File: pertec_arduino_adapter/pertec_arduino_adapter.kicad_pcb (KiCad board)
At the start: 2 copper layers, 88.9 x 78.7 mm, 19 parts, among them J1 Conn_02x25_Odd_Even, J2 Conn_02x25_Odd_Even, J3 POWER, J4 ANALOGL, J5 ANALOGH, J6 Conn_02x18_Odd_Even, J7 IOH, J8 IOL, J9 UART, U1 SN74AVC8T245PW, U2 SN74AVC8T245PW, U3 SN74AVC8T245PW, U4 SN74AVC8T245PW, U5 SN74AVC8T245PW, U6 SN74AVC8T245PW

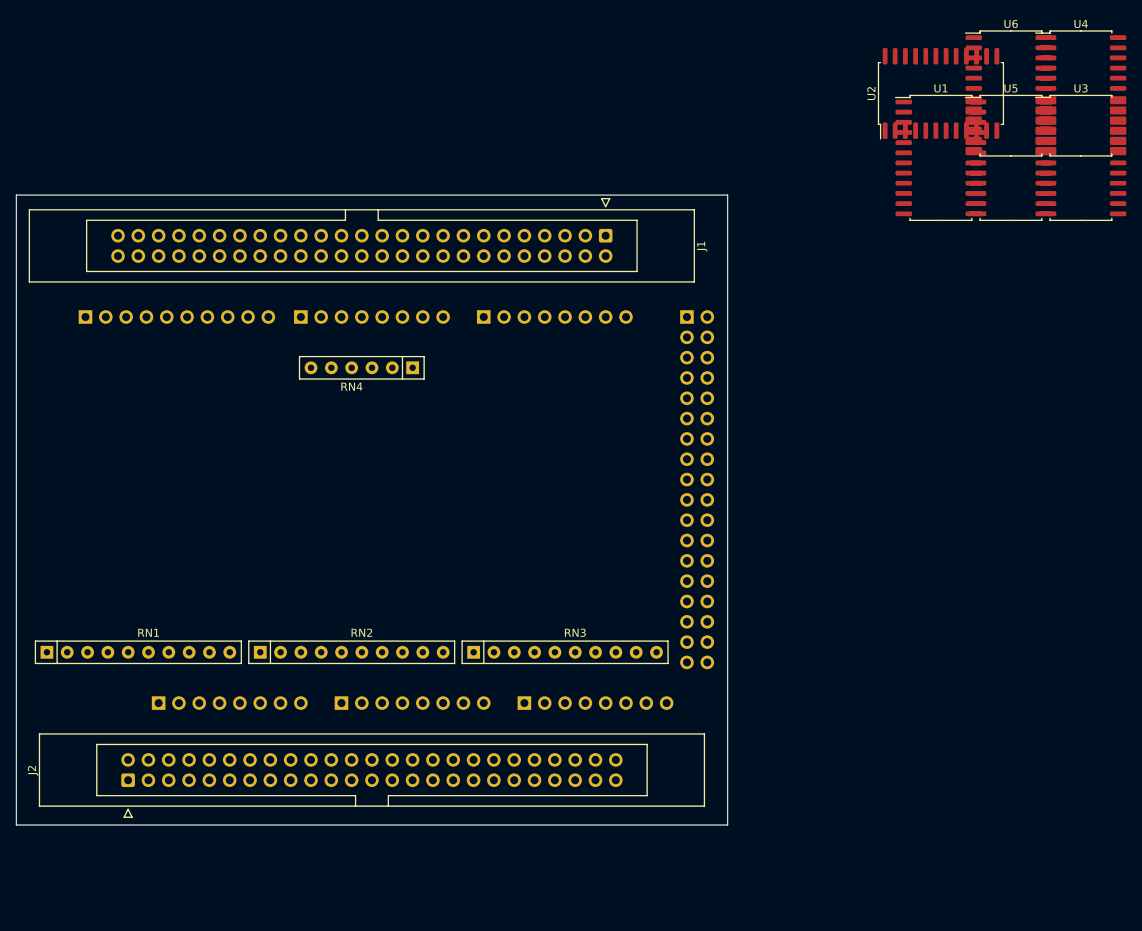
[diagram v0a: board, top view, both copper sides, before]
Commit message: Development checkpoint: schematic complete, passes ERC, started layout.
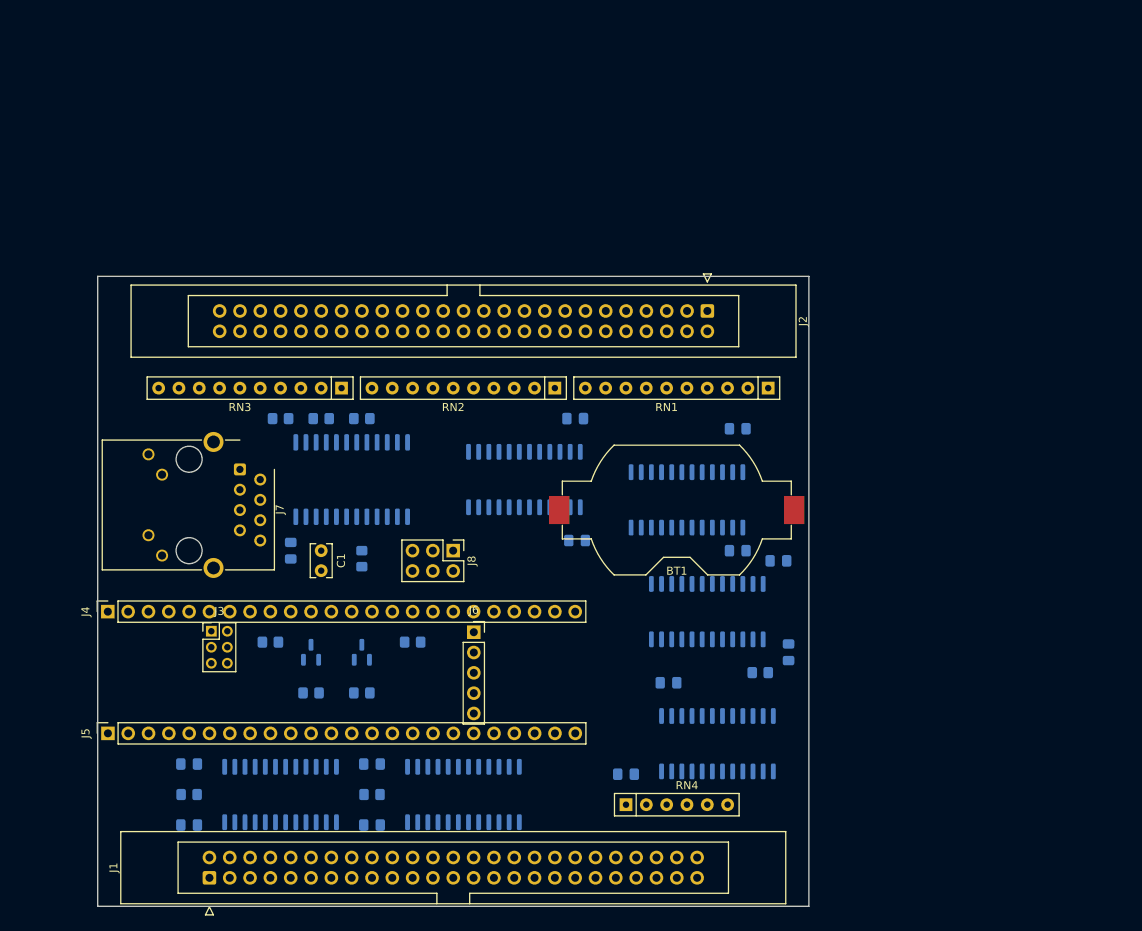
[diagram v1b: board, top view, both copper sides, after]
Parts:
- removed J9: UART, pertec_arduino_adapter:PinHeader_1x08_P2.54mm_Vertical
- added BT1: CR2032, pertec_arduino_adapter:BatteryHolder_Keystone_1058_1x2032, F.Cu at (158.8, 74.9)
- added C1: 0.1 μF, pertec_arduino_adapter:C_Rect_L4.0mm_W2.5mm_P2.50mm, F.Cu at (114.3, 80.0)
- added C10: 0.1 μF, pertec_arduino_adapter:C_0805_2012Metric_Pad1.18x1.45mm_HandSolder, B.Cu at (97.8, 114.3)
- added C11: 0.1 μF, pertec_arduino_adapter:C_0805_2012Metric_Pad1.18x1.45mm_HandSolder, B.Cu at (157.7, 96.5)
- added C12: 0.1 μF, pertec_arduino_adapter:C_0805_2012Metric_Pad1.18x1.45mm_HandSolder, B.Cu at (171.4, 81.3)
- added C13: 0.1 μF, pertec_arduino_adapter:C_0805_2012Metric_Pad1.18x1.45mm_HandSolder, B.Cu at (172.7, 92.7)
- added C14: 0.1 μF, pertec_arduino_adapter:C_0805_2012Metric_Pad1.18x1.45mm_HandSolder, B.Cu at (166.4, 64.8)
- added C2: 0.1 μF, pertec_arduino_adapter:C_0805_2012Metric_Pad1.18x1.45mm_HandSolder, B.Cu at (110.5, 80.0)
- added C3: 0.1 μF, pertec_arduino_adapter:C_0805_2012Metric_Pad1.18x1.45mm_HandSolder, B.Cu at (97.8, 106.7)
- added C4: 0.1 μF, pertec_arduino_adapter:C_0805_2012Metric_Pad1.18x1.45mm_HandSolder, B.Cu at (146.1, 63.5)
- added C5: 0.1 μF, pertec_arduino_adapter:C_0805_2012Metric_Pad1.18x1.45mm_HandSolder, B.Cu at (146.3, 78.7)
- added C6: 0.1 μF, pertec_arduino_adapter:C_0805_2012Metric_Pad1.18x1.45mm_HandSolder, B.Cu at (152.4, 108.0)
- added C7: 0.1 μF, pertec_arduino_adapter:C_0805_2012Metric_Pad1.18x1.45mm_HandSolder, B.Cu at (120.7, 106.7)
- added C8: 0.1 μF, pertec_arduino_adapter:C_0805_2012Metric_Pad1.18x1.45mm_HandSolder, B.Cu at (120.7, 114.3)
- added C9: 0.1 μF, pertec_arduino_adapter:C_0805_2012Metric_Pad1.18x1.45mm_HandSolder, B.Cu at (166.4, 80.0)
- added Q1: BSS138, pertec_arduino_adapter:SOT-23, B.Cu at (113.0, 92.7)
- added Q2: BSS138, pertec_arduino_adapter:SOT-23, B.Cu at (119.4, 92.7)
- added R1: 10 kΩ, pertec_arduino_adapter:R_0805_2012Metric_Pad1.20x1.40mm_HandSolder, B.Cu at (113.0, 97.8)
- added R10: 10 kΩ, pertec_arduino_adapter:R_0805_2012Metric_Pad1.20x1.40mm_HandSolder, B.Cu at (120.7, 110.5)
- added R11: 10 kΩ, pertec_arduino_adapter:R_0805_2012Metric_Pad1.20x1.40mm_HandSolder, B.Cu at (169.2, 95.2)
- added R2: 10 kΩ, pertec_arduino_adapter:R_0805_2012Metric_Pad1.20x1.40mm_HandSolder, B.Cu at (119.4, 97.8)
- added R3: 10 kΩ, pertec_arduino_adapter:R_0805_2012Metric_Pad1.20x1.40mm_HandSolder, B.Cu at (108.0, 91.4)
- added R4: 10 kΩ, pertec_arduino_adapter:R_0805_2012Metric_Pad1.20x1.40mm_HandSolder, B.Cu at (125.7, 91.4)
- added R5: 10 kΩ, pertec_arduino_adapter:R_0805_2012Metric_Pad1.20x1.40mm_HandSolder, B.Cu at (119.4, 63.5)
- added R6: 10 kΩ, pertec_arduino_adapter:R_0805_2012Metric_Pad1.20x1.40mm_HandSolder, B.Cu at (114.3, 63.5)
- added R7: 10 kΩ, pertec_arduino_adapter:R_0805_2012Metric_Pad1.20x1.40mm_HandSolder, B.Cu at (109.2, 63.5)
- added R8: 10 kΩ, pertec_arduino_adapter:R_0805_2012Metric_Pad1.20x1.40mm_HandSolder, B.Cu at (119.4, 81.0)
- added R9: 10 kΩ, pertec_arduino_adapter:R_0805_2012Metric_Pad1.20x1.40mm_HandSolder, B.Cu at (97.8, 110.5)
- added U7: PCA9535DBR, pertec_arduino_adapter:SOIC-24W_7.5x15.4mm_P1.27mm, B.Cu at (118.1, 71.1)
- J3: value POWER -> Conn_02x03_Odd_Even; footprint pertec_arduino_adapter:PinHeader_1x08_P2.54mm_Vertical -> pertec_arduino_adapter:PinSocket_2x03_P2.00mm_Vertical_Mirror; moved to F.Cu
- J4: value ANALOGL -> Conn_01x24; footprint pertec_arduino_adapter:PinHeader_1x08_P2.54mm_Vertical -> pertec_arduino_adapter:PinSocket_1x24_P2.54mm_Vertical; moved to F.Cu
- J5: value ANALOGH -> Conn_01x24; footprint pertec_arduino_adapter:PinHeader_1x08_P2.54mm_Vertical -> pertec_arduino_adapter:PinSocket_1x24_P2.54mm_Vertical; moved to F.Cu
- J6: value Conn_02x18_Odd_Even -> Conn_01x05; footprint pertec_arduino_adapter:PinHeader_2x18_P2.54mm_Vertical_Mirror -> pertec_arduino_adapter:PinSocket_1x05_P2.54mm_Vertical; moved to F.Cu
- J7: value IOH -> RJ45_Cetus_J1B1211CCD; footprint pertec_arduino_adapter:PinHeader_1x10_P2.54mm_Vertical -> pertec_arduino_adapter:RJ45_Cetus_J1B1211CCD_Horizontal; moved to F.Cu
- J8: value IOL -> Conn_02x03_Odd_Even; footprint pertec_arduino_adapter:PinHeader_1x08_P2.54mm_Vertical -> pertec_arduino_adapter:PinHeader_2x03_P2.54mm_Vertical; moved to F.Cu
- U1, U2, U3, U4, U5, U6: value SN74AVC8T245PW -> SN74LVC8T245NSR; footprint pertec_arduino_adapter:SOIC-24W_7.5x15.4mm_P1.27mm -> pertec_arduino_adapter:SO-24_5.3x15mm_P1.27mm; moved to B.Cu
- moved U2 120.4 mm to (109.2, 110.5), turned to -90 degrees
- moved U4 116.8 mm to (132.1, 110.5), turned to -90 degrees
- moved RN1 96.0 mm to (170.2, 59.7), turned to 180 degrees
- moved J1 94.3 mm to (100.3, 120.9), turned to 90 degrees
- moved J2 93.2 mm to (162.6, 50.0), turned to -90 degrees
- moved U5 81.9 mm to (163.8, 104.1), turned to -90 degrees
- moved U3 80.4 mm to (139.7, 71.1), turned to 90 degrees
- moved U6 75.1 mm to (162.6, 87.6), turned to 90 degrees
- moved RN4 60.8 mm to (152.4, 111.8), turned to 0 degrees
- moved U1 53.3 mm to (160.0, 73.7), turned to 90 degrees
- moved J5 52.2 mm to (87.6, 102.8), turned to 90 degrees
- moved RN2 49.5 mm to (143.5, 59.7), turned to 180 degrees
- moved J6 47.6 mm to (133.4, 90.2), turned to 0 degrees
- moved RN3 36.9 mm to (116.8, 59.7), turned to 180 degrees
- moved J8 34.9 mm to (130.8, 80.0)
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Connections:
- J2 pad 50: IHISP -> IDEN
- J3 pad 1: unconnected-(J3-Pad1) -> ETHERNET_TM
- J3 pad 2: +3V3 -> ETHERNET_TP
- J3 pad 3: ~{RESET} -> ETHERNET_LED
- J3 pad 4: +3V3 -> ETHERNET_G
- J3 pad 5: +5V -> ETHERNET_RP
- J3 pad 6: GNDREF -> ETHERNET_RM
- J4 pad 1: A0 -> +5V
- J4 pad 2: A1 -> GNDREF
- J4 pad 3: A2 -> +3V3
- J4 pad 4: A3 -> GPIO_AD_B1_09
- J4 pad 5: A4 -> GPIO_AD_B1_08
- J4 pad 6: A5 -> GPIO_AD_B1_11
- J4 pad 7: A6 -> GPIO_AD_B1_10
- J4 pad 8: A7 -> GPIO_AD_B1_00
- J5 pad 1: A8 -> GNDREF
- J5 pad 2: A9 -> GPIO_AD_B0_03
- J5 pad 3: A10 -> GPIO_AD_B0_02
- J5 pad 4: A11 -> GPIO_EMC_04
- J5 pad 5: A12 -> GPIO_EMC_05
- J5 pad 6: A13 -> GPIO_EMC_06
- J5 pad 7: A14 -> GPIO_EMC_08
- J5 pad 8: A15 -> GPIO_B0_10
- J6 pad 1: +5V -> unconnected-(J6-Pad1)
- J6 pad 2: +5V -> unconnected-(J6-Pad2)
- J6 pad 3: D22 -> GNDREF
- J6 pad 4: A10 -> unconnected-(J6-Pad4)
- J6 pad 5: SCL_1 -> Net-(BT1-Pad1)
- J7 pad 1: SCL -> ETHERNET_TP
- J7 pad 10: D8 -> ETHERNET_LED
- J7 pad 2: SDA -> Net-(J7-Pad2)
- J7 pad 3: AREF -> ETHERNET_TM
- J7 pad 4: GND -> ETHERNET_RP
- J7 pad 5: D13 -> Net-(J7-Pad2)
- J7 pad 6: D12 -> ETHERNET_RM
- J7 pad 7: D11 -> unconnected-(J7-Pad7)
- J7 pad 8: D10 -> ETHERNET_G
- J7 pad 9: D9 -> ETHERNET_G
- J8 pad 1: D7 -> GNDREF
- J8 pad 2: D6 -> SPARE0
- J8 pad 3: D5 -> GNDREF
- J8 pad 4: D4 -> SPARE1
- J8 pad 5: D3 -> GNDREF
- J8 pad 6: D2 -> GPIO_EMC_31
- U1 pad 1: unconnected-(U1-Pad1) -> +3V3
- U1 pad 10: unconnected-(U1-Pad10) -> GPIO_B1_12
- U1 pad 11: Net-(U1-Pad11) -> GNDREF
- U1 pad 12: Net-(U1-Pad11) -> GNDREF
- U1 pad 13: Net-(U1-Pad11) -> GNDREF
- U1 pad 14: unconnected-(U1-Pad14) -> IHER
- U1 pad 15: unconnected-(U1-Pad15) -> IR6
- U1 pad 16: unconnected-(U1-Pad16) -> IR7
- U1 pad 17: unconnected-(U1-Pad17) -> IR4
- U1 pad 18: unconnected-(U1-Pad18) -> ILDP
- U1 pad 19: unconnected-(U1-Pad19) -> IR1
- U1 pad 2: unconnected-(U1-Pad2) -> GNDREF
- U1 pad 20: unconnected-(U1-Pad20) -> IR0
- U1 pad 21: unconnected-(U1-Pad21) -> IRP
- U1 pad 22: unconnected-(U1-Pad22) -> GNDREF
- U1 pad 23: unconnected-(U1-Pad23) -> +5V
- U1 pad 24: unconnected-(U1-Pad24) -> +5V
- U1 pad 3: unconnected-(U1-Pad3) -> GPIO_AD_B0_02
- U1 pad 4: unconnected-(U1-Pad4) -> GPIO_AD_B1_07
- U1 pad 5: unconnected-(U1-Pad5) -> GPIO_AD_B1_06
- U1 pad 6: unconnected-(U1-Pad6) -> GPIO_EMC_32
- U1 pad 7: unconnected-(U1-Pad7) -> GPIO_AD_B1_03
- U1 pad 8: unconnected-(U1-Pad8) -> GPIO_AD_B1_00
- U1 pad 9: unconnected-(U1-Pad9) -> GPIO_AD_B1_01
- U2 pad 1: unconnected-(U2-Pad1) -> +3V3
- U2 pad 10: unconnected-(U2-Pad10) -> GPIO_B1_01
- U2 pad 11: Net-(U2-Pad11) -> GNDREF
- U2 pad 12: Net-(U2-Pad11) -> GNDREF
- U2 pad 13: Net-(U2-Pad11) -> GNDREF
- U2 pad 14: unconnected-(U2-Pad14) -> IWP
- U2 pad 15: unconnected-(U2-Pad15) -> IREW
- U2 pad 16: unconnected-(U2-Pad16) -> IREV
- U2 pad 17: unconnected-(U2-Pad17) -> IW1
- U2 pad 18: unconnected-(U2-Pad18) -> IW0
- U2 pad 19: unconnected-(U2-Pad19) -> IGO
- U2 pad 2: unconnected-(U2-Pad2) -> Net-(U2-Pad2)
- U2 pad 20: unconnected-(U2-Pad20) -> IW4
- U2 pad 21: unconnected-(U2-Pad21) -> ILWD
- U2 pad 22: unconnected-(U2-Pad22) -> GNDREF
- U2 pad 23: unconnected-(U2-Pad23) -> +5V
- U2 pad 24: unconnected-(U2-Pad24) -> +5V
- U2 pad 3: unconnected-(U2-Pad3) -> GPIO_B0_03
- U2 pad 4: unconnected-(U2-Pad4) -> GPIO_AD_B1_11
- U2 pad 5: unconnected-(U2-Pad5) -> GPIO_B0_10
- U2 pad 6: unconnected-(U2-Pad6) -> GPIO_AD_B1_15
- U2 pad 7: unconnected-(U2-Pad7) -> GPIO_AD_B1_14
- U2 pad 8: unconnected-(U2-Pad8) -> GPIO_B0_11
- U2 pad 9: unconnected-(U2-Pad9) -> GPIO_B1_00
- U3 pad 1: unconnected-(U3-Pad1) -> +3V3
- U3 pad 10: unconnected-(U3-Pad10) -> GPIO_EMC_06
- U3 pad 11: Net-(U3-Pad11) -> GNDREF
- U3 pad 12: Net-(U3-Pad11) -> GNDREF
- U3 pad 13: Net-(U3-Pad11) -> GNDREF
- U3 pad 14: unconnected-(U3-Pad14) -> IDBY
- U3 pad 15: unconnected-(U3-Pad15) -> IWSTR
- U3 pad 16: unconnected-(U3-Pad16) -> IRSTR
- U3 pad 17: unconnected-(U3-Pad17) -> IFPT
- U3 pad 18: unconnected-(U3-Pad18) -> IRDY
- U3 pad 19: unconnected-(U3-Pad19) -> IEOT
- U3 pad 2: unconnected-(U3-Pad2) -> GNDREF
- U3 pad 20: unconnected-(U3-Pad20) -> IR5
- U3 pad 21: unconnected-(U3-Pad21) -> IFMK
- U3 pad 22: unconnected-(U3-Pad22) -> GNDREF
- U3 pad 23: unconnected-(U3-Pad23) -> +5V
- U3 pad 24: unconnected-(U3-Pad24) -> +5V
- U3 pad 3: unconnected-(U3-Pad3) -> GPIO_AD_B0_03
- U3 pad 4: unconnected-(U3-Pad4) -> GPIO_AD_B1_02
- U3 pad 5: unconnected-(U3-Pad5) -> GPIO_EMC_36
- U3 pad 6: unconnected-(U3-Pad6) -> GPIO_EMC_04
- U3 pad 7: unconnected-(U3-Pad7) -> GPIO_EMC_05
- U3 pad 8: unconnected-(U3-Pad8) -> GPIO_B1_02
- U3 pad 9: unconnected-(U3-Pad9) -> GPIO_B1_03
- U4 pad 1: unconnected-(U4-Pad1) -> +3V3
- U4 pad 10: unconnected-(U4-Pad10) -> GPIO_B0_01
- U4 pad 11: Net-(U4-Pad11) -> GNDREF
- U4 pad 12: Net-(U4-Pad11) -> GNDREF
- U4 pad 13: Net-(U4-Pad11) -> GNDREF
- U4 pad 14: unconnected-(U4-Pad14) -> IERASE
- U4 pad 15: unconnected-(U4-Pad15) -> IEDIT
- U4 pad 16: unconnected-(U4-Pad16) -> IWRT
- U4 pad 17: unconnected-(U4-Pad17) -> IW5
- U4 pad 18: unconnected-(U4-Pad18) -> IW2
- U4 pad 19: unconnected-(U4-Pad19) -> IW6
- U4 pad 2: unconnected-(U4-Pad2) -> Net-(U4-Pad2)
- U4 pad 20: unconnected-(U4-Pad20) -> IW3
- U4 pad 21: unconnected-(U4-Pad21) -> IW7
- U4 pad 22: unconnected-(U4-Pad22) -> GNDREF
- U4 pad 23: unconnected-(U4-Pad23) -> +5V
- U4 pad 24: unconnected-(U4-Pad24) -> +5V
- U4 pad 3: unconnected-(U4-Pad3) -> GPIO_AD_B1_08
- U4 pad 4: unconnected-(U4-Pad4) -> GPIO_AD_B1_12
- U4 pad 5: unconnected-(U4-Pad5) -> GPIO_AD_B1_09
- U4 pad 6: unconnected-(U4-Pad6) -> GPIO_AD_B1_13
- U4 pad 7: unconnected-(U4-Pad7) -> GPIO_AD_B1_10
- U4 pad 8: unconnected-(U4-Pad8) -> GPIO_B0_00
- U4 pad 9: unconnected-(U4-Pad9) -> GPIO_B0_02
- U5 pad 1: unconnected-(U5-Pad1) -> +3V3
- U5 pad 11: Net-(U5-Pad11) -> GNDREF
- U5 pad 12: Net-(U5-Pad11) -> GNDREF
- U5 pad 13: Net-(U5-Pad11) -> GNDREF
- U5 pad 18: unconnected-(U5-Pad18) -> IR3
- U5 pad 19: unconnected-(U5-Pad19) -> IR2
- U5 pad 2: unconnected-(U5-Pad2) -> GNDREF
- U5 pad 20: unconnected-(U5-Pad20) -> IFBY
- U5 pad 21: unconnected-(U5-Pad21) -> ICER
- U5 pad 22: unconnected-(U5-Pad22) -> GNDREF
- U5 pad 23: unconnected-(U5-Pad23) -> +5V
- U5 pad 24: unconnected-(U5-Pad24) -> +5V
- U5 pad 3: unconnected-(U5-Pad3) -> GPIO_B1_13
- U5 pad 4: unconnected-(U5-Pad4) -> GPIO_EMC_07
- U5 pad 5: unconnected-(U5-Pad5) -> GPIO_AD_B1_05
- U5 pad 6: unconnected-(U5-Pad6) -> GPIO_AD_B1_04
- U6 pad 1: unconnected-(U6-Pad1) -> +3V3
- U6 pad 10: unconnected-(U6-Pad10) -> GPIO_EMC_37
- U6 pad 11: Net-(U6-Pad11) -> GNDREF
- U6 pad 12: Net-(U6-Pad11) -> GNDREF
- U6 pad 13: Net-(U6-Pad11) -> GNDREF
- U6 pad 14: unconnected-(U6-Pad14) -> IOFL
- U6 pad 15: unconnected-(U6-Pad15) -> IWFM
- U6 pad 2: unconnected-(U6-Pad2) -> Net-(U6-Pad2)
- U6 pad 22: unconnected-(U6-Pad22) -> GNDREF
- U6 pad 23: unconnected-(U6-Pad23) -> +5V
- U6 pad 24: unconnected-(U6-Pad24) -> +5V
- U6 pad 9: unconnected-(U6-Pad9) -> GPIO_B0_12
